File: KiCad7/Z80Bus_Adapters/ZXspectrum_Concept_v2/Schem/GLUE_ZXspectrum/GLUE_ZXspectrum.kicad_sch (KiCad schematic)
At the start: 14 parts

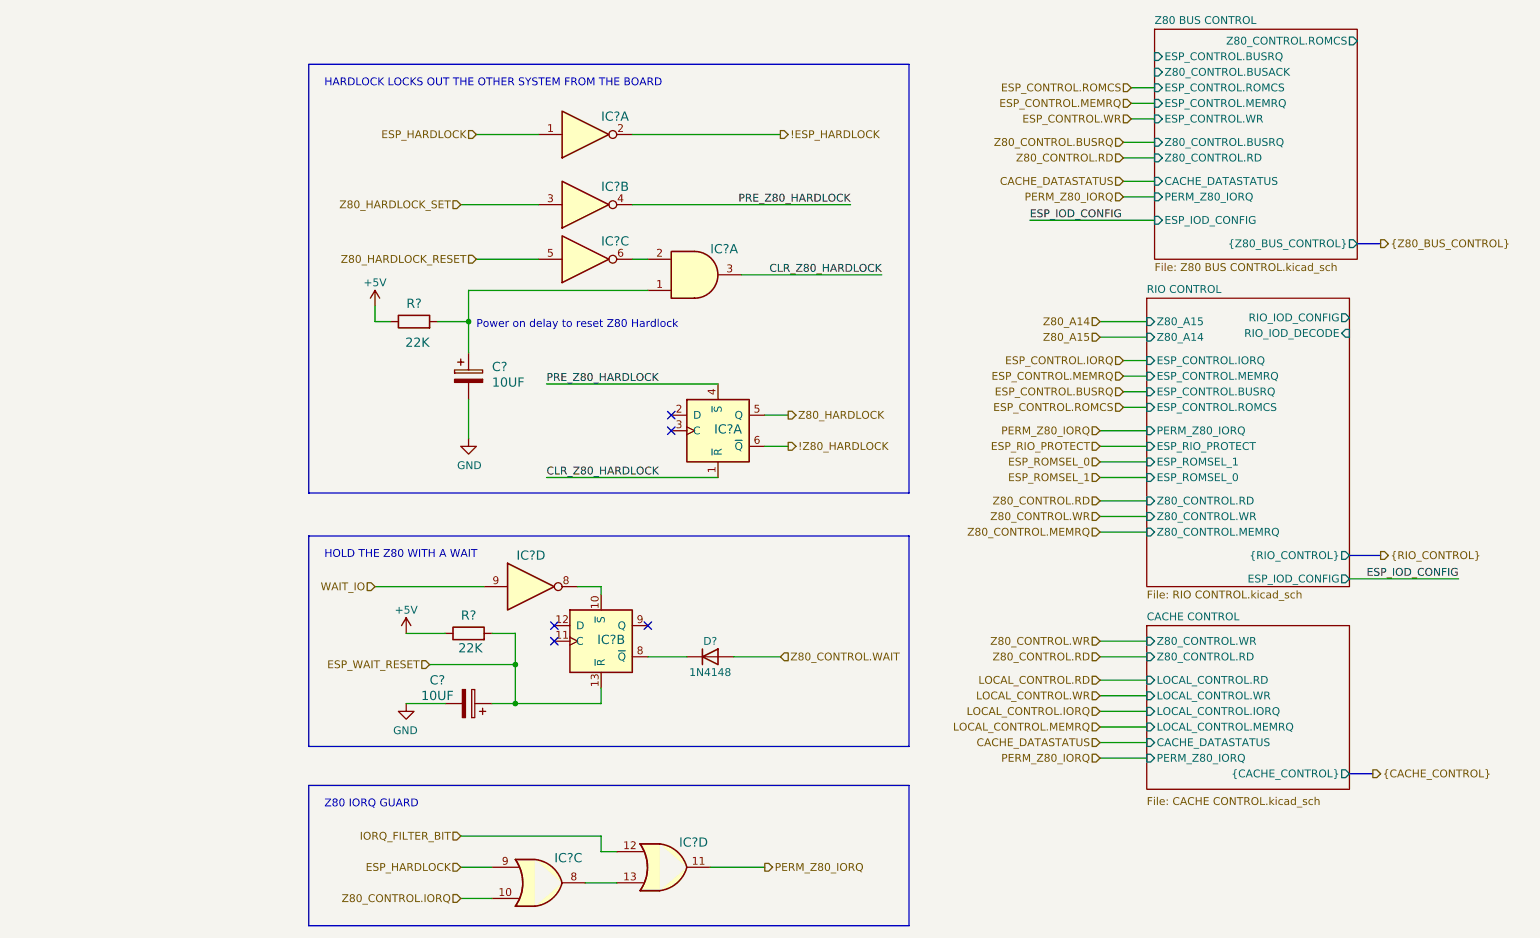
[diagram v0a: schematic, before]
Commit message: ThatOldNerds V2 of the concept design.
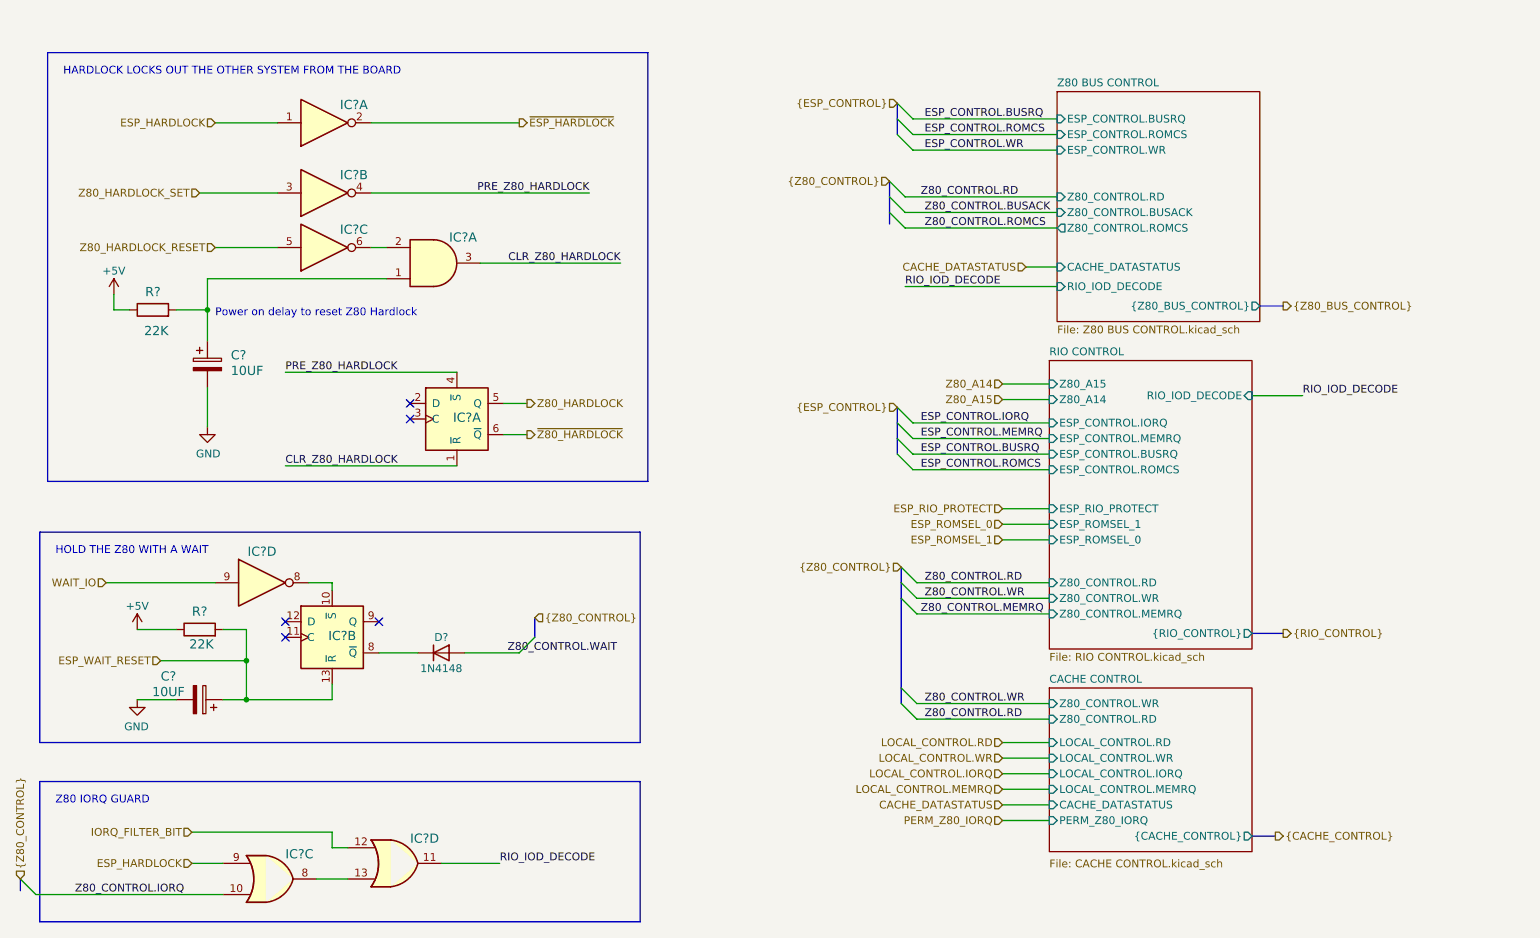
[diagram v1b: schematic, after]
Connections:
- net PERM_Z80_IORQ: no longer IC?.11
- net !ESP_HARDLOCK renamed ~{ESP_HARDLOCK}
- net !Z80_HARDLOCK renamed ~{Z80_HARDLOCK}
- new net RIO_IOD_DECODE: IC?.11
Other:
- sheet RIO CONTROL ports: added none; removed ESP_IOD_CONFIG, PERM_Z80_IORQ, RIO_IOD_CONFIG
- sheet Z80 BUS CONTROL ports: added RIO_IOD_DECODE; removed ESP_CONTROL.MEMRQ, ESP_IOD_CONFIG, PERM_Z80_IORQ, Z80_CONTROL.BUSRQ
- moved on the sheet: C?, D?, IC?A, IC?B, IC?C, IC?D, R?
